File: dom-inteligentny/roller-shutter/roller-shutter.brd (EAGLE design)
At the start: 64 x 84 mm, 19 parts, among them K1 RP421110, K2 691218410003, K3 691218410003, K4 RP421110, Q1 16MHz, T1 BC847, T2 BC847, U1 ATMEGA328

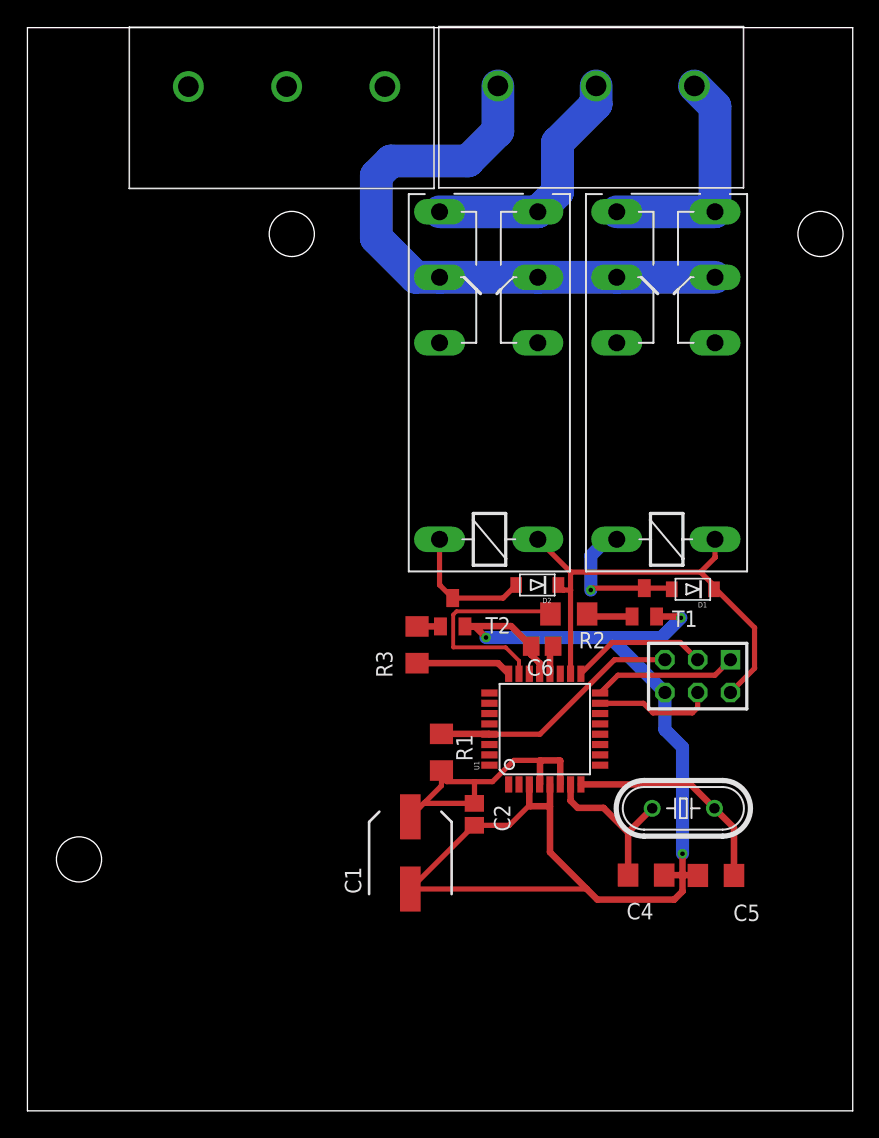
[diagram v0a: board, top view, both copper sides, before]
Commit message: Roller shutter
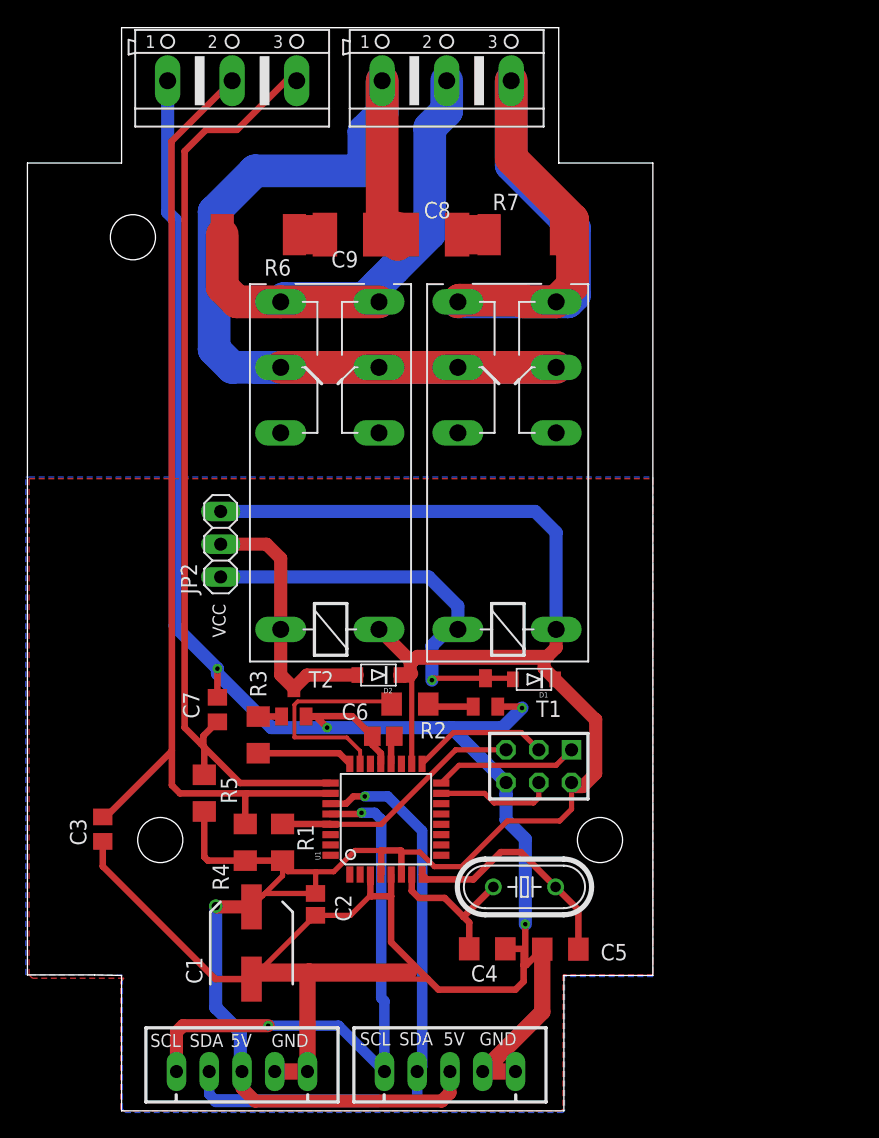
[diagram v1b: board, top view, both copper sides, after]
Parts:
- removed K2, K3: 691218410003, Wurth_Elektronik_Electromechanic_Terminal_Blocks_Connectors_rev15c:691218410003
- added C3, C7: (no value), eagle-ltspice:C0805
- added C8, C9: (no value), eagle-ltspice:C1812
- added JP2: (no value), pinhead:1X03
- added R4, R5: (no value), eagle-ltspice:R1206
- added R6, R7: (no value), eagle-ltspice:R2512
- added X1, X4: (no value), con-ptr500:AK500/3
- added X2, X3: JST-XH-05-PIN-LONG-PAD, Rembrandt Electronics - JST XH Connectors v1-0:JST-XH-05-PACKAGE-LONG-PAD
- moved JP1 14.2 mm to (39.7, 26.7)
- moved K4 14.2 mm to (23.5, 41.1)
- moved R2 14.2 mm to (29.7, 31.5)
- moved D2 14.2 mm to (27.2, 33.8)
- moved R3 14.2 mm to (17.9, 29.2)
- moved C1 14.2 mm to (17.4, 13.0)
- moved C2 14.2 mm to (22.3, 16.0)
- moved U1 14.2 mm to (27.8, 22.6)
- moved D1 14.2 mm to (39.3, 33.5)
- moved K1 14.2 mm to (37.2, 41.1)
- moved R1 14.2 mm to (19.8, 20.8)
- moved T1 14.2 mm to (35.5, 32.4)
- moved T2 14.2 mm to (20.7, 31.7)
- moved C6 14.2 mm to (27.6, 29.1)
- moved Q1 13.7 mm to (38.5, 17.4)
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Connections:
- new net N$10: C9.2, R6.1
- new net N$9: C8.2, R7.1
- net A2: now also C7.2, R5.1, X4.3
- net A3: now also C3.2, R4.1, X4.2
- net A4: now also X2.2, X3.2
- net A5: now also X2.1, X3.1
- net GND: now also C3.1, C7.1, X2.4, X2.5, X3.4, X3.5, X4.1
- net N$1: now also JP2.1
- net N$2: now also JP2.2
- net N$4: now also C8.1, C9.1, X1.1; no longer K3.1
- net N$7: now also R7.2, X1.3; no longer K3.3
- net N$8: now also R6.2, X1.2; no longer K3.2
- net VCC: now also JP2.3, R4.2, R5.2, X2.3, X3.3
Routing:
- net GND: track 98.7 -> 218.7 mm, vias 3 -> 4
- net VCC: track 61.9 -> 176.9 mm, vias 0 -> 1
- net A3: track 0.00 -> 79.1 mm
- net A2: track 0.00 -> 73.3 mm
- net N$4: track 46.7 -> 98.5 mm
- net A4: track 0.00 -> 47.6 mm, vias 0 -> 1
- net A5: track 0.00 -> 44.7 mm, vias 0 -> 2
- net N$7: track 18.0 -> 61.4 mm
- net N$8: track 19.3 -> 44.2 mm
- net N$1: track 11.6 -> 32.7 mm
- net N$2: track 10.3 -> 20.9 mm
- net N$9: track 0.00 -> 2.49 mm
- net N$10: track 0.00 -> 2.36 mm
- net N$44: track 17.0 -> 18.3 mm
- net N$43: track 12.7 -> 12.1 mm
- added copper zone on layer 1, net GND
- added copper zone on layer 16, net GND
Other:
- board size 64 x 84 mm -> 48.5 x 84 mm
- board text added: "5V"
- board text added: "Falcon IoT Roller Shutter v1.0 weblogic.pl falcon.software"
- board text added: "GND"
- board text added: "SCL"
- board text added: "SDA"
- board text added: "VCC"
